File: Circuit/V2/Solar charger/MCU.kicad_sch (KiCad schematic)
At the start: 1 part

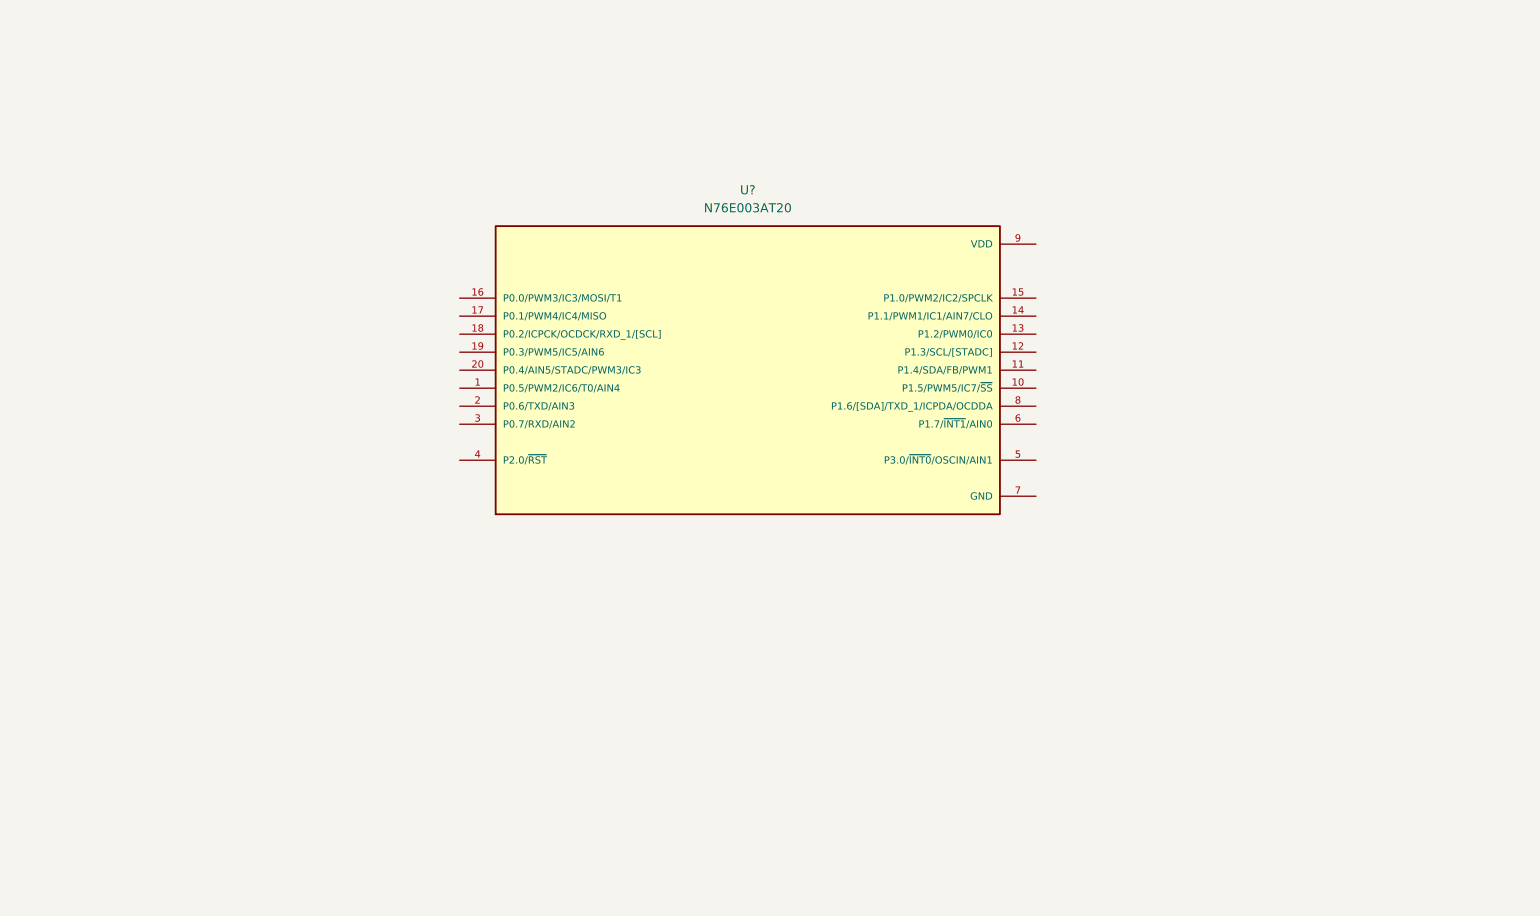
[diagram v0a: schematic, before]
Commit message: update
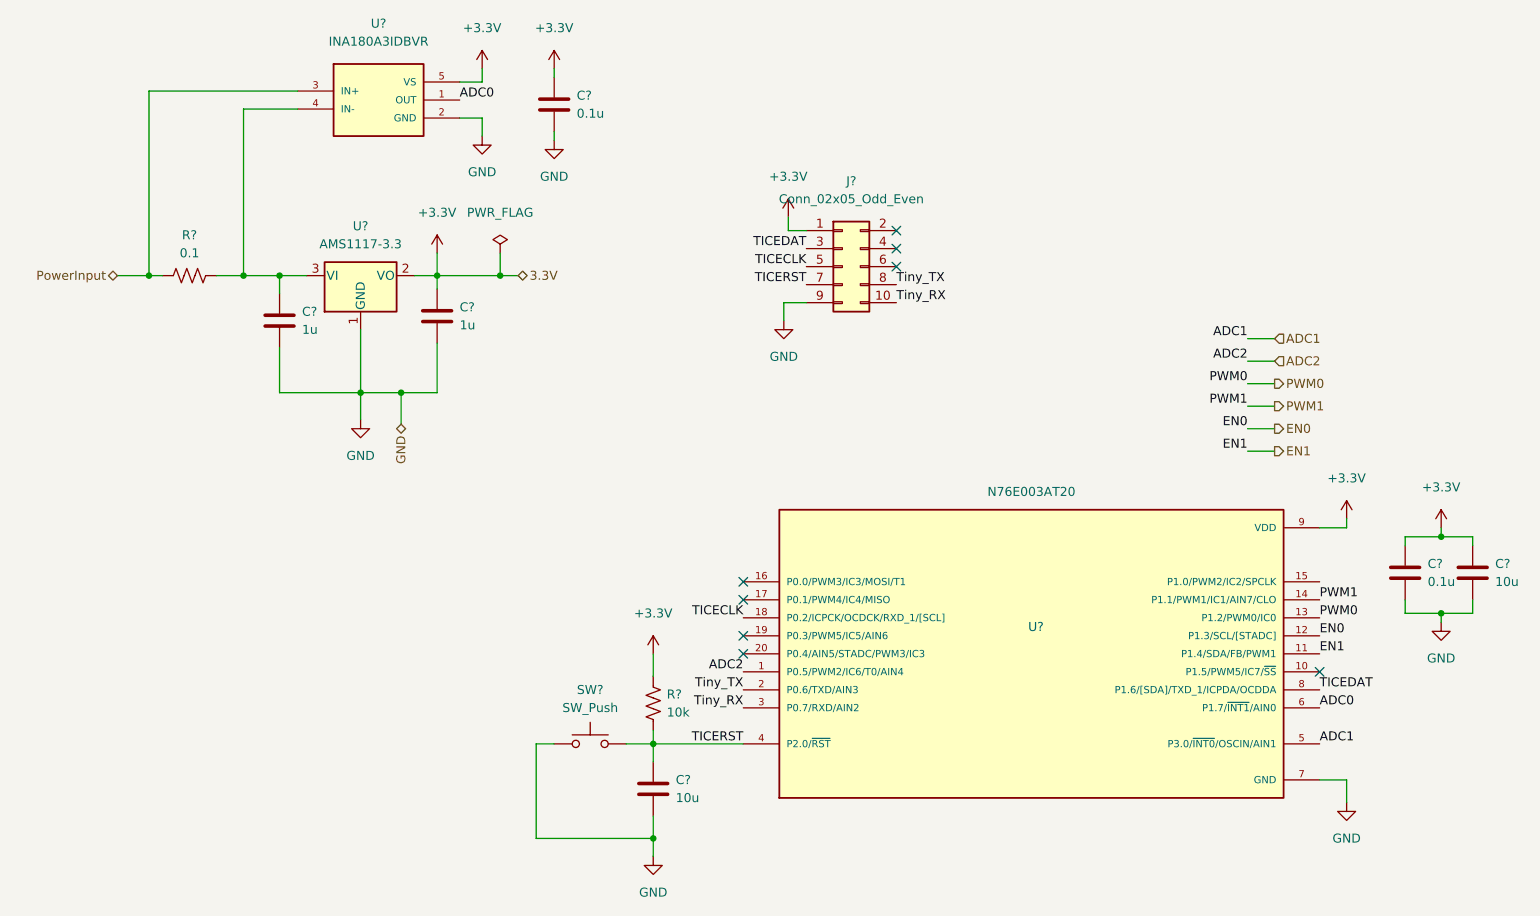
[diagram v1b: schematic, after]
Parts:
- added C? (x2): 0.1u, Capacitor_SMD:C_0805_2012Metric, symbol 1CommonUse:C0805
- added C? (x2): 10u, Capacitor_SMD:C_0805_2012Metric, symbol 1CommonUse:C0805
- added C? (x2): 1u, Capacitor_SMD:C_0805_2012Metric, symbol 1CommonUse:C0805
- added J?: Conn_02x05_Odd_Even, Connector_IDC:IDC-Header_2x05_P2.54mm_Vertical, symbol Connector_Generic:Conn_02x05_Odd_Even
- added R?: 0.1, Resistor_SMD:R_0805_2012Metric, symbol 1CommonUse:R0805
- added R?: 10k, Resistor_SMD:R_0805_2012Metric, symbol 1CommonUse:R0805
- added SW?: SW_Push, symbol Switch:SW_Push
- added U?: INA180A3IDBVR, Package_TO_SOT_SMD:SOT-23-5, symbol SolarCharger:INA180A3IDBVR
- added U?: AMS1117-3.3, Package_TO_SOT_SMD:SOT-223-3_TabPin2, symbol Regulator_Linear:AMS1117-3.3
- U?: footprint SolarCharger:SOP65P640X120-20N -> Package_SO:TSSOP-20_4.4x6.5mm_P0.65mm
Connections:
- net ADC2: now reaches U?.1 (P0.5/PWM2/IC6/T0/AIN4)
- net EN1: now reaches U?.11 (P1.4/SDA/FB/PWM1)
- net EN0: now reaches U?.12 (P1.3/SCL/[STADC])
- net PWM0: now reaches U?.13 (P1.2/PWM0/IC0)
- net PWM1: now reaches U?.14 (P1.1/PWM1/IC1/AIN7/CLO)
- net TICECLK: now reaches U?.18 (P0.2/ICPCK/OCDCK/RXD_1/[SCL])
- net TICECLK: now also J?.5 (Pin_5)
- net Tiny_TX: now reaches U?.2 (P0.6/TXD/AIN3)
- net Tiny_TX: now also J?.8 (Pin_8)
- net Tiny_RX: now reaches U?.3 (P0.7/RXD/AIN2)
- net Tiny_RX: now also J?.10 (Pin_10)
- net TICERST: now reaches U?.4 (P2.0/~{RST})
- net TICERST: now also C?.1, J?.7 (Pin_7), R?.2, SW?.2
- net ADC1: now reaches U?.5 (P3.0/~{INT0}/OSCIN/AIN1)
- net ADC0: now reaches U?.6 (P1.7/~{INT1}/AIN0)
- net ADC0: now also U?.1 (OUT)
- net GND: now reaches U?.7 (GND)
- net GND: now also C?.2, C?.2, C?.2, C?.2, C?.2, C?.2, J?.9 (Pin_9), SW?.1, U?.1 (GND), U?.2 (GND)
- net TICEDAT: now reaches U?.8 (P1.6/[SDA]/TXD_1/ICPDA/OCDDA)
- net TICEDAT: now also J?.3 (Pin_3)
- net +3.3V: now reaches U?.9 (VDD)
- net +3.3V: now also C?.1, C?.1, C?.1, C?.1, J?.1 (Pin_1), R?.1, U?.2 (VO), U?.5 (VS)
- new net: C?.1, R?.2, U?.3 (VI), U?.4 (IN-)
- new net PowerInput: R?.1, U?.3 (IN+)
- no-connect marks 0 -> 8
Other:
- moved on the sheet: U?
